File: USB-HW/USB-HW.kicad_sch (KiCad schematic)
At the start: 21 parts, among them J1 USB A, U1 SP0503BAHTG, U2 CP2102

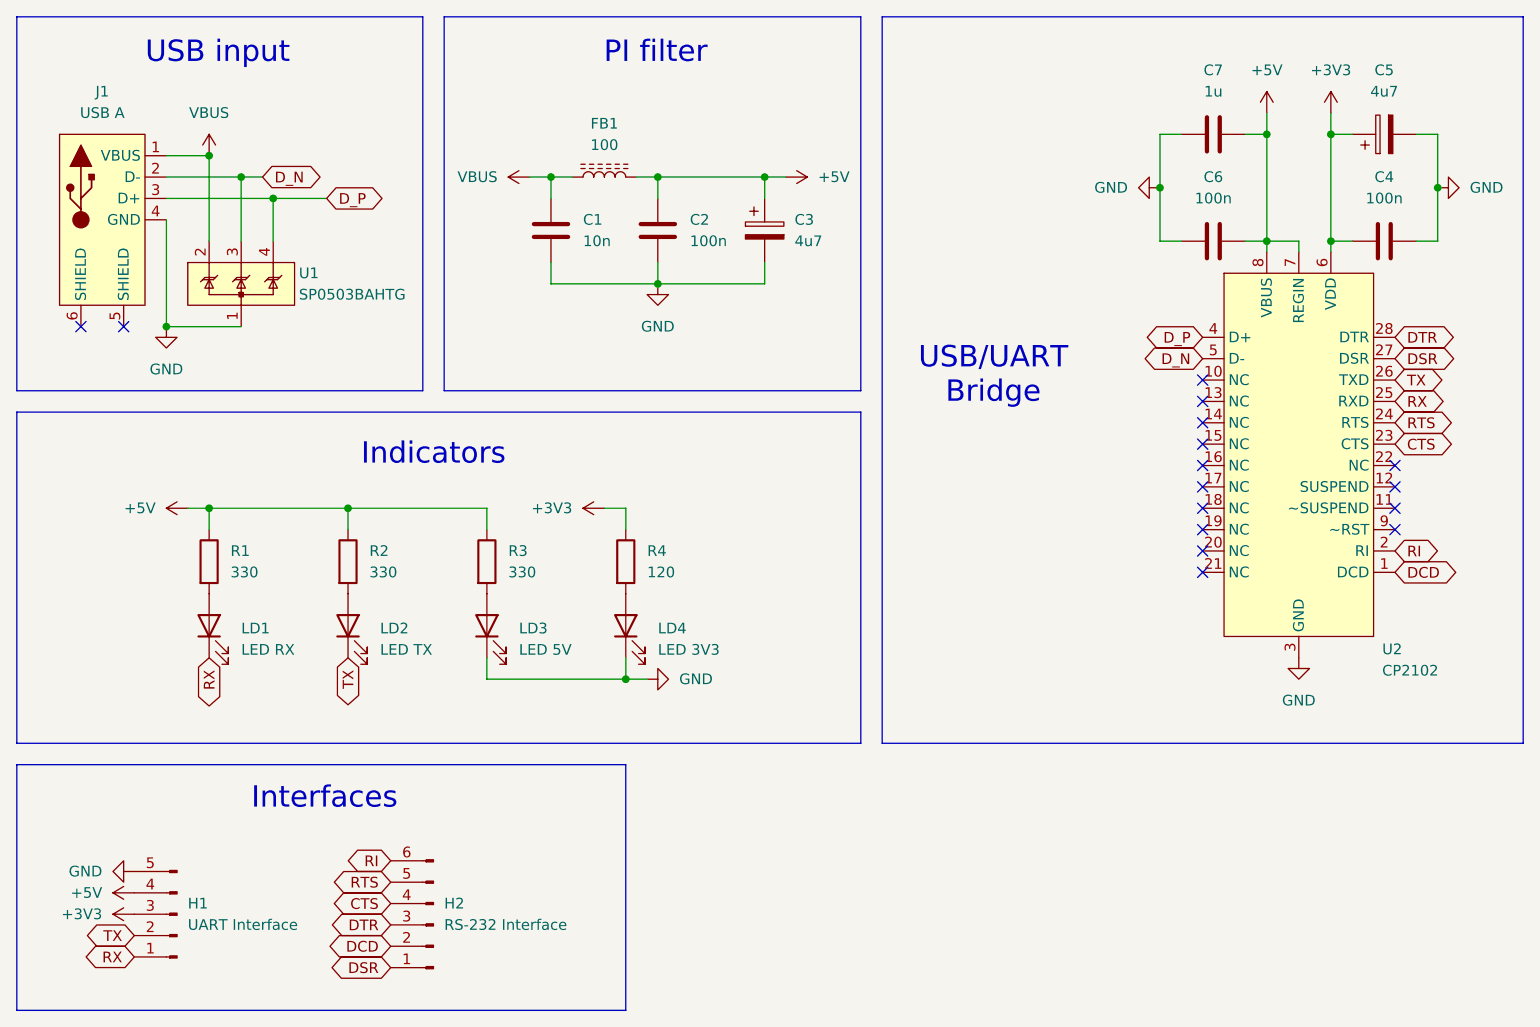
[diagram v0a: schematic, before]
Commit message: feat: Add footprints
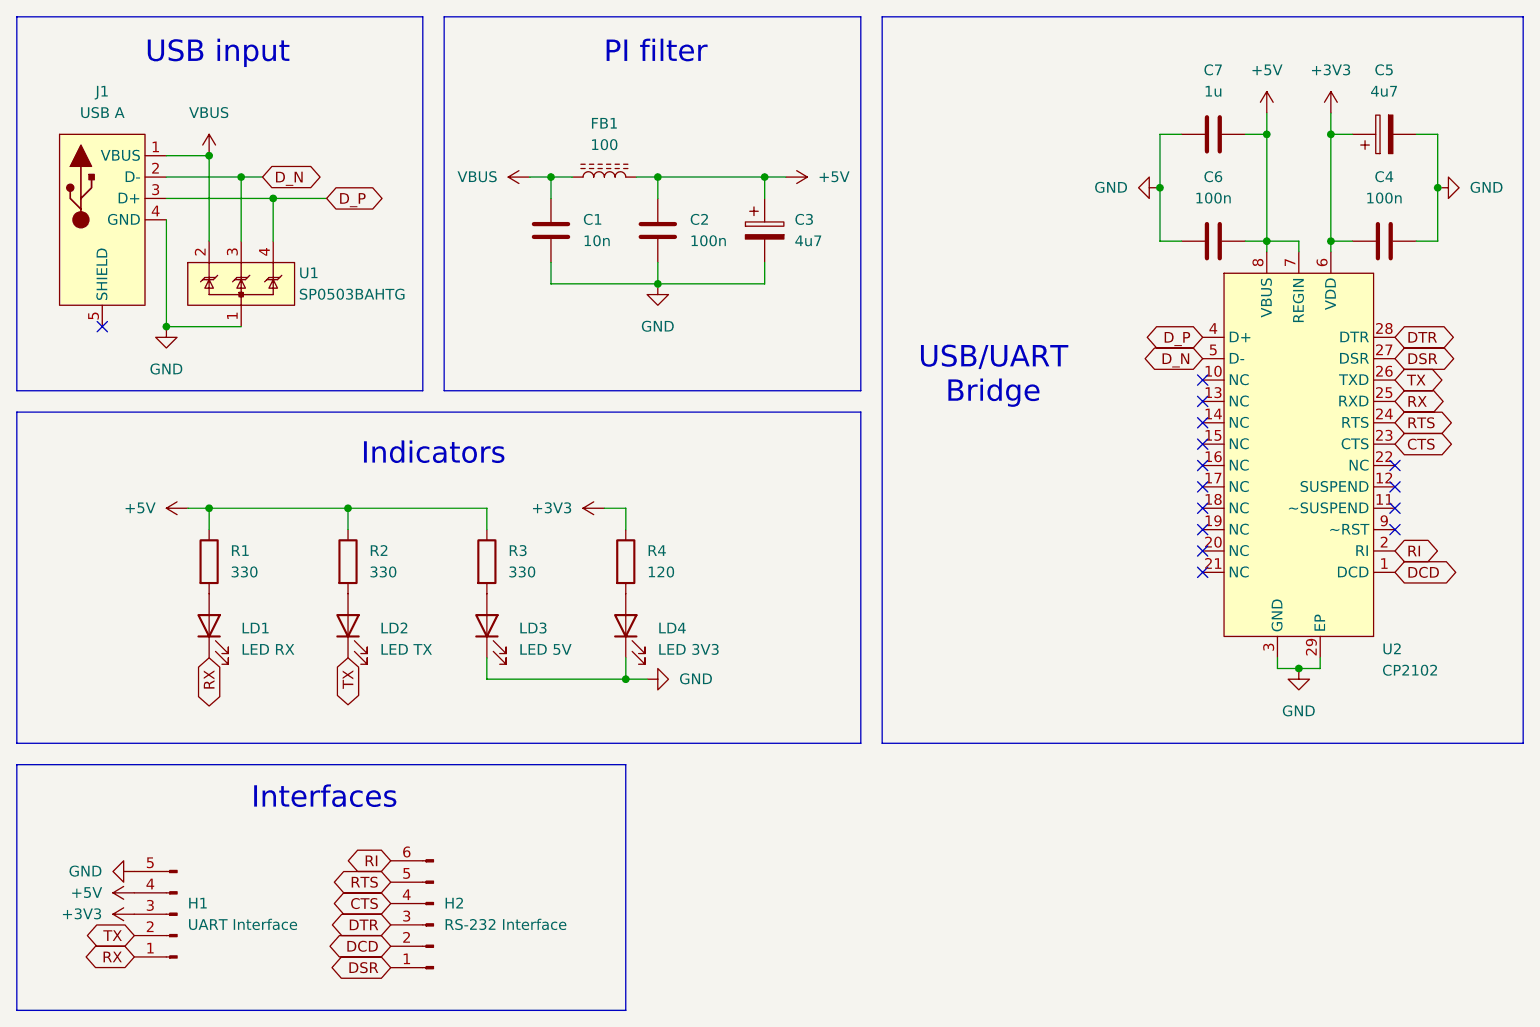
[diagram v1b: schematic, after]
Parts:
- C1, C2, C4, C6, C7: footprint (none) -> Capacitor_SMD:C_0805_2012Metric
- C3, C5: footprint (none) -> Capacitor_SMD:CP_Elec_4x5.3
- FB1: footprint (none) -> Inductor_SMD:L_0805_2012Metric
- H1: footprint (none) -> Connector_PinHeader_2.54mm:PinHeader_1x05_P2.54mm_Vertical
- H2: footprint (none) -> Connector_PinSocket_2.54mm:PinSocket_1x06_P2.54mm_Vertical
- J1: footprint (none) -> Connector_USB:USB_A_Molex_48037-2200_Horizontal
- LD1, LD2, LD3, LD4: footprint (none) -> LED_SMD:LED_0805_2012Metric
- R1, R2, R3, R4: footprint (none) -> Resistor_SMD:R_0805_2012Metric
- U1: footprint (none) -> Package_TO_SOT_SMD:SOT-143
- U2: footprint (none) -> Package_DFN_QFN:QFN-28-1EP_5x5mm_P0.5mm_EP3.25x3.25mm
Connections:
- net GND: now also U2.29 (EP)
- no-connect marks 16 -> 15
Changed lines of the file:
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@@
 	)
 	(junction
+		(at 167.64 92.71)
+		(diameter 0)
+		(color 0 0 0 0)
+	)
+	(junction
 		(at 45.72 36.83)
 		(diameter 0)
@@
 	)
 	(no_connect
-		(at 27.94 52.07)
+		(at 25.4 52.07)
 	)
 	(no_connect
@@
 	)
 	(no_connect
-		(at 22.86 52.07)
-	)
-	(no_connect
 		(at 156.21 66.04)
 	)
@@
 	(wire
 		(pts
+			(xy 170.18 92.71) (xy 170.18 91.44)
+		)
+		(stroke
+			(width 0)
+			(type default)
+		)
+	)
+	(wire
+		(pts
 			(xy 71.12 73.66) (xy 71.12 76.2)
 		)
@@
 	(wire
 		(pts
+			(xy 165.1 92.71) (xy 165.1 91.44)
+		)
+		(stroke
+			(width 0)
+			(type default)
+		)
+	)
+	(wire
+		(pts
 			(xy 90.17 93.98) (xy 87.63 93.98)
 		)
@@
 	(wire
 		(pts
+			(xy 167.64 92.71) (xy 170.18 92.71)
+		)
+		(stroke
+			(width 0)
+			(type default)
+		)
+	)
+	(wire
+		(pts
 			(xy 104.14 36.83) (xy 104.14 34.29)
 		)
@@
 	(wire
 		(pts
+			(xy 167.64 92.71) (xy 165.1 92.71)
+		)
+		(stroke
+			(width 0)
+			(type default)
+		)
+	)
+	(wire
+		(pts
 			(xy 161.29 41.91) (xy 163.83 41.91)
 		)
@@
 			)
 		)
-		(property "Footprint" ""
+		(property "Footprint" "Resistor_SMD:R_0805_2012Metric"
 			(at 36.322 80.01 90)
 			(effects
@@
 			)
 		)
-		(property "Footprint" ""
+		(property "Footprint" "Connector_PinSocket_2.54mm:PinSocket_1x06_P2.54mm_Vertical"
 			(at 64.77 123.19 0)
 			(effects
@@
 			)
 		)
-		(property "Footprint" ""
+		(property "Footprint" "Resistor_SMD:R_0805_2012Metric"
 			(at 52.832 80.01 90)
 			(effects
@@
 			)
 		)
-		(property "Footprint" ""
+		(property "Footprint" "Capacitor_SMD:C_0805_2012Metric"
 			(at 153.67 42.8752 0)
 			(effects
@@
 			)
 		)
-		(property "Footprint" ""
+		(property "Footprint" "Capacitor_SMD:CP_Elec_4x5.3"
 			(at 105.1052 44.45 0)
 			(effects
@@
 			)
 		)
-		(property "Footprint" ""
+		(property "Footprint" "Resistor_SMD:R_0805_2012Metric"
 			(at 85.852 80.01 90)
 			(effects
@@
 			)
 		)
-		(property "Footprint" ""
+		(property "Footprint" "Capacitor_SMD:CP_Elec_4x5.3"
 			(at 181.61 28.2448 0)
 			(effects
@@
 			)
 		)
-		(property "Footprint" ""
+		(property "Footprint" "Capacitor_SMD:C_0805_2012Metric"
 			(at 92.4052 44.45 0)
 			(effects
@@
 	(symbol
 		(lib_id "power:GND")
-		(at 167.64 91.44 0)
+		(at 167.64 92.71 0)
 		(unit 1)
 		(exclude_from_sim no)
@@
 		(fields_autoplaced yes)
 		(property "Reference" "#PWR06"
-			(at 167.64 97.79 0)
+			(at 167.64 99.06 0)
 			(effects
 				(font
@@
 		)
 		(property "Value" "GND"
-			(at 167.64 96.52 0)
+			(at 167.64 97.79 0)
 			(effects
 				(font
@@
 		)
 		(property "Footprint" ""
-			(at 167.64 91.44 0)
+			(at 167.64 92.71 0)
 			(effects
 				(font
@@
 		)
 		(property "Datasheet" ""
-			(at 167.64 91.44 0)
+			(at 167.64 92.71 0)
 			(effects
 				(font
@@
 		)
 		(property "Description" "Power symbol creates a global label with name \"GND\" , ground"
-			(at 167.64 91.44 0)
+			(at 167.64 92.71 0)
 			(effects
 				(font
@@
 			)
 		)
-		(property "Footprint" ""
+		(property "Footprint" "Capacitor_SMD:C_0805_2012Metric"
 			(at 153.67 30.1752 0)
 			(effects
@@
 			)
 		)
-		(property "Footprint" ""
+		(property "Footprint" "LED_SMD:LED_0805_2012Metric"
 			(at 54.61 87.63 0)
 			(effects
@@
 			)
 		)
-		(property "Footprint" ""
+		(property "Footprint" "Package_TO_SOT_SMD:SOT-143"
 			(at 41.91 46.99 0)
 			(effects
@@
 			)
 		)
-		(property "Footprint" ""
+		(property "Footprint" "Connector_USB:USB_A_Molex_48037-2200_Horizontal"
 			(at 25.4 39.37 0)
 			(effects
@@
 		(pin "1"
 		)
-		(pin "6"
-		)
 		(pin "3"
 		)
@@
 			)
 		)
-		(property "Footprint" ""
+		(property "Footprint" "LED_SMD:LED_0805_2012Metric"
 			(at 87.63 87.63 0)
 			(effects
@@
 			)
 		)
-		(property "Footprint" ""
+		(property "Footprint" "Capacitor_SMD:C_0805_2012Metric"
 			(at 173.99 42.8752 0)
 			(effects
@@
 			)
 		)
-		(property "Footprint" ""
+		(property "Footprint" "Inductor_SMD:L_0805_2012Metric"
 			(at 85.09 34.29 0)
 			(effects
@@
 			)
 		)
-		(property "Footprint" ""
+		(property "Footprint" "Package_DFN_QFN:QFN-28-1EP_5x5mm_P0.5mm_EP3.25x3.25mm"
 			(at 167.64 64.77 0)
 			(effects
@@
 		(pin "18"
 		)
+		(pin "29"
+		)
 		(instances
 			(project ""
@@
 			)
 		)
-		(property "Footprint" ""
+		(property "Footprint" "Connector_PinHeader_2.54mm:PinHeader_1x05_P2.54mm_Vertical"
 			(at 34.29 121.92 0)
 			(effects
@@
 			)
 		)
-		(property "Footprint" ""
+		(property "Footprint" "LED_SMD:LED_0805_2012Metric"
 			(at 71.12 87.63 0)
 			(effects
@@
 			)
 		)
-		(property "Footprint" ""
+		(property "Footprint" "Capacitor_SMD:C_0805_2012Metric"
 			(at 79.7052 44.45 0)
 			(effects
@@
 			)
 		)
-		(property "Footprint" ""
+		(property "Footprint" "LED_SMD:LED_0805_2012Metric"
 			(at 38.1 87.63 0)
 			(effects
@@
 			)
 		)
-		(property "Footprint" ""
+		(property "Footprint" "Resistor_SMD:R_0805_2012Metric"
 			(at 69.342 80.01 90)
 			(effects

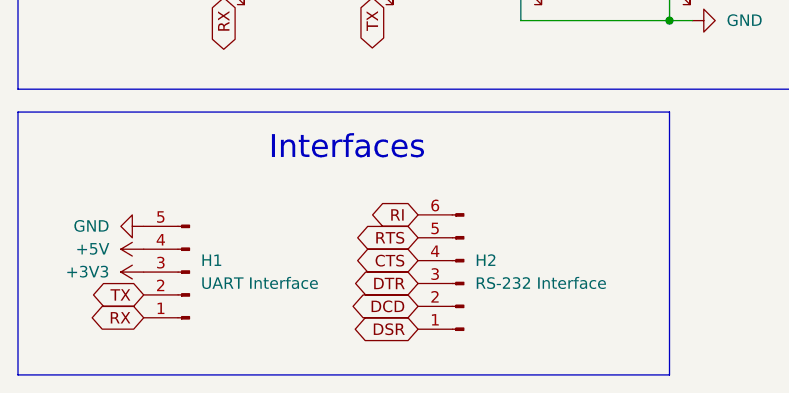
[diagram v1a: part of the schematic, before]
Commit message: feat: Add PCB
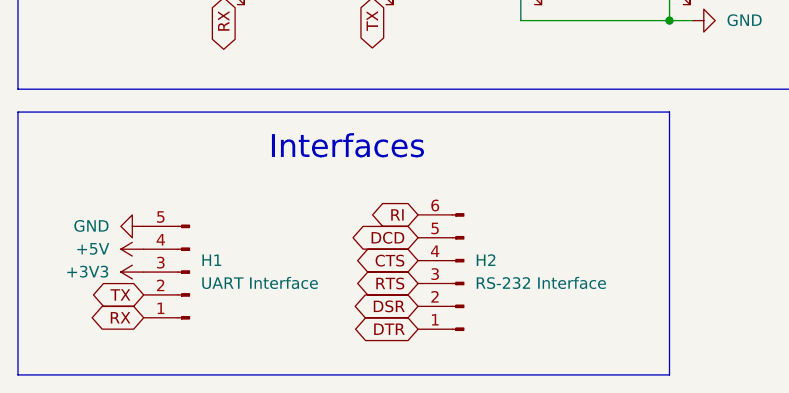
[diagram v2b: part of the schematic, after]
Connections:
- net DCD: now also H2.5 (Pin_5); no longer H2.2 (Pin_2)
- net DSR: now also H2.2 (Pin_2); no longer H2.1 (Pin_1)
- net DTR: now also H2.1 (Pin_1); no longer H2.3 (Pin_3)
- net RTS: now also H2.3 (Pin_3); no longer H2.5 (Pin_5)
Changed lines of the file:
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@@
 	(global_label "RTS"
 		(shape bidirectional)
+		(at 59.69 123.19 180)
+		(fields_autoplaced yes)
+		(effects
+			(font
+				(size 1.27 1.27)
+			)
+			(justify right)
+		)
+		(property "Intersheetrefs" "${INTERSHEET_REFS}"
+			(at 52.1464 123.19 0)
+			(effects
+				(font
+					(size 1.27 1.27)
+				)
+				(justify right)
+				(hide yes)
+			)
+		)
+	)
+	(global_label "DCD"
+		(shape bidirectional)
+		(at 179.07 81.28 0)
+		(fields_autoplaced yes)
+		(effects
+			(font
+				(size 1.27 1.27)
+			)
+			(justify left)
+		)
+		(property "Intersheetrefs" "${INTERSHEET_REFS}"
+			(at 186.9765 81.28 0)
+			(effects
+				(font
+					(size 1.27 1.27)
+				)
+				(justify left)
+				(hide yes)
+			)
+		)
+	)
+	(global_label "RTS"
+		(shape bidirectional)
+		(at 179.07 63.5 0)
+		(fields_autoplaced yes)
+		(effects
+			(font
+				(size 1.27 1.27)
+			)
+			(justify left)
+		)
+		(property "Intersheetrefs" "${INTERSHEET_REFS}"
+			(at 186.6136 63.5 0)
+			(effects
+				(font
+					(size 1.27 1.27)
+				)
+				(justify left)
+				(hide yes)
+			)
+		)
+	)
+	(global_label "TX"
+		(shape bidirectional)
+		(at 54.61 91.44 270)
+		(fields_autoplaced yes)
+		(effects
+			(font
+				(size 1.27 1.27)
+			)
+			(justify right)
+		)
+		(property "Intersheetrefs" "${INTERSHEET_REFS}"
+			(at 54.61 97.7136 90)
+			(effects
+				(font
+					(size 1.27 1.27)
+				)
+				(justify right)
+				(hide yes)
+			)
+		)
+	)
+	(global_label "RX"
+		(shape bidirectional)
+		(at 179.07 60.96 0)
+		(effects
+			(font
+				(size 1.27 1.27)
+			)
+			(justify left)
+		)
+		(property "Intersheetrefs" "${INTERSHEET_REFS}"
+			(at 186.6136 60.96 0)
+			(effects
+				(font
+					(size 1.27 1.27)
+				)
+				(justify left)
+				(hide yes)
+			)
+		)
+	)
+	(global_label "D_P"
+		(shape bidirectional)
+		(at 156.21 53.34 180)
+		(fields_autoplaced yes)
+		(effects
+			(font
+				(size 1.27 1.27)
+			)
+			(justify right)
+		)
+		(property "Intersheetrefs" "${INTERSHEET_REFS}"
+			(at 148.6059 53.34 0)
+			(effects
+				(font
+					(size 1.27 1.27)
+				)
+				(justify right)
+				(hide yes)
+			)
+		)
+	)
+	(global_label "D_N"
+		(shape bidirectional)
+		(at 156.21 55.88 180)
+		(fields_autoplaced yes)
+		(effects
+			(font
+				(size 1.27 1.27)
+			)
+			(justify right)
+		)
+		(property "Intersheetrefs" "${INTERSHEET_REFS}"
+			(at 148.5454 55.88 0)
+			(effects
+				(font
+					(size 1.27 1.27)
+				)
+				(justify right)
+				(hide yes)
+			)
+		)
+	)
+	(global_label "DTR"
+		(shape bidirectional)
+		(at 59.69 128.27 180)
+		(fields_autoplaced yes)
+		(effects
+			(font
+				(size 1.27 1.27)
+			)
+			(justify right)
+		)
+		(property "Intersheetrefs" "${INTERSHEET_REFS}"
+			(at 52.0859 128.27 0)
+			(effects
+				(font
+					(size 1.27 1.27)
+				)
+				(justify right)
+				(hide yes)
+			)
+		)
+	)
+	(global_label "DSR"
+		(shape bidirectional)
+		(at 59.69 125.73 180)
+		(fields_autoplaced yes)
+		(effects
+			(font
+				(size 1.27 1.27)
+			)
+			(justify right)
+		)
+		(property "Intersheetrefs" "${INTERSHEET_REFS}"
+			(at 51.844 125.73 0)
+			(effects
+				(font
+					(size 1.27 1.27)
+				)
+				(justify right)
+				(hide yes)
+			)
+		)
+	)
+	(global_label "DCD"
+		(shape bidirectional)
 		(at 59.69 118.11 180)
 		(fields_autoplaced yes)
@@
 		)
 		(property "Intersheetrefs" "${INTERSHEET_REFS}"
-			(at 52.1464 118.11 0)
-			(effects
-				(font
-					(size 1.27 1.27)
-				)
-				(justify right)
-				(hide yes)
-			)
-		)
-	)
-	(global_label "DCD"
-		(shape bidirectional)
-		(at 179.07 81.28 0)
-		(fields_autoplaced yes)
-		(effects
-			(font
-				(size 1.27 1.27)
-			)
-			(justify left)
-		)
-		(property "Intersheetrefs" "${INTERSHEET_REFS}"
-			(at 186.9765 81.28 0)
-			(effects
-				(font
-					(size 1.27 1.27)
-				)
-				(justify left)
-				(hide yes)
-			)
-		)
-	)
-	(global_label "RTS"
-		(shape bidirectional)
-		(at 179.07 63.5 0)
-		(fields_autoplaced yes)
-		(effects
-			(font
-				(size 1.27 1.27)
-			)
-			(justify left)
-		)
-		(property "Intersheetrefs" "${INTERSHEET_REFS}"
-			(at 186.6136 63.5 0)
-			(effects
-				(font
-					(size 1.27 1.27)
-				)
-				(justify left)
-				(hide yes)
-			)
-		)
-	)
-	(global_label "TX"
-		(shape bidirectional)
-		(at 54.61 91.44 270)
-		(fields_autoplaced yes)
-		(effects
-			(font
-				(size 1.27 1.27)
-			)
-			(justify right)
-		)
-		(property "Intersheetrefs" "${INTERSHEET_REFS}"
-			(at 54.61 97.7136 90)
-			(effects
-				(font
-					(size 1.27 1.27)
-				)
-				(justify right)
-				(hide yes)
-			)
-		)
-	)
-	(global_label "RX"
-		(shape bidirectional)
-		(at 179.07 60.96 0)
-		(effects
-			(font
-				(size 1.27 1.27)
-			)
-			(justify left)
-		)
-		(property "Intersheetrefs" "${INTERSHEET_REFS}"
-			(at 186.6136 60.96 0)
-			(effects
-				(font
-					(size 1.27 1.27)
-				)
-				(justify left)
-				(hide yes)
-			)
-		)
-	)
-	(global_label "D_P"
-		(shape bidirectional)
-		(at 156.21 53.34 180)
-		(fields_autoplaced yes)
-		(effects
-			(font
-				(size 1.27 1.27)
-			)
-			(justify right)
-		)
-		(property "Intersheetrefs" "${INTERSHEET_REFS}"
-			(at 148.6059 53.34 0)
-			(effects
-				(font
-					(size 1.27 1.27)
-				)
-				(justify right)
-				(hide yes)
-			)
-		)
-	)
-	(global_label "D_N"
-		(shape bidirectional)
-		(at 156.21 55.88 180)
-		(fields_autoplaced yes)
-		(effects
-			(font
-				(size 1.27 1.27)
-			)
-			(justify right)
-		)
-		(property "Intersheetrefs" "${INTERSHEET_REFS}"
-			(at 148.5454 55.88 0)
-			(effects
-				(font
-					(size 1.27 1.27)
-				)
-				(justify right)
-				(hide yes)
-			)
-		)
-	)
-	(global_label "DTR"
-		(shape bidirectional)
-		(at 59.69 123.19 180)
-		(fields_autoplaced yes)
-		(effects
-			(font
-				(size 1.27 1.27)
-			)
-			(justify right)
-		)
-		(property "Intersheetrefs" "${INTERSHEET_REFS}"
-			(at 52.0859 123.19 0)
-			(effects
-				(font
-					(size 1.27 1.27)
-				)
-				(justify right)
-				(hide yes)
-			)
-		)
-	)
-	(global_label "DSR"
-		(shape bidirectional)
-		(at 59.69 128.27 180)
-		(fields_autoplaced yes)
-		(effects
-			(font
-				(size 1.27 1.27)
-			)
-			(justify right)
-		)
-		(property "Intersheetrefs" "${INTERSHEET_REFS}"
-			(at 51.844 128.27 0)
-			(effects
-				(font
-					(size 1.27 1.27)
-				)
-				(justify right)
-				(hide yes)
-			)
-		)
-	)
-	(global_label "DCD"
-		(shape bidirectional)
-		(at 59.69 125.73 180)
-		(fields_autoplaced yes)
-		(effects
-			(font
-				(size 1.27 1.27)
-			)
-			(justify right)
-		)
-		(property "Intersheetrefs" "${INTERSHEET_REFS}"
-			(at 51.7835 125.73 0)
-			(effects
-				(font
+			(at 51.7835 118.11 0)
+			(effects
+				(font
